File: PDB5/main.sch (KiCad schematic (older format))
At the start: 31 parts, among them P1 CONN_02X03, P4 CONN_01X02, P5 CONN_01X10, P6 CONN_01X10, P7 CONN_01X10, U1 PCA9698, U10 LTC6802-2, U11 LTC6802-2, U12 LTC6802-2, U13 LTC6802-2, U7 Littlebee, U8 Littlebee, U9 SC18IS602B

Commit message: test
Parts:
- removed P? (x3): CONN_01X03, symbol CONN_01X03
- removed R?: R, symbol R
- removed U10, U11, U12, U13: LTC6802-2, symbol LTC6802-2
- added C1: C, Capacitors_SMD:C_0805, symbol C
- added D1: ZENER, Diodes_SMD:SOD-123, symbol ZENER
- added D3: LED, LEDs:LED_0603, symbol LED
- added P10, P2, P3, P7, P8, P9: CONN_01X02, Pin_Headers:Pin_Header_Straight_1x02, symbol CONN_01X02
- added P15, P16: CONN_XT60_Female, KiCad-Dev:XT60, symbol CONN_XT60_Female
- added R2: R, Resistors_SMD:R_0603, symbol R
- added R3: R, symbol R
- C2: renamed from C?; footprint (none) -> SMD_Packages:SMD-2010_Pol
- C3: renamed from C?; footprint (none) -> Capacitors_SMD:C_0805
- D2: renamed from D?; footprint (none) -> LEDs:LED_0603
- D4: renamed from D?; footprint (none) -> Diodes_SMD:SOD-123
- P1: renamed from P?; footprint (none) -> Pin_Headers:Pin_Header_Straight_1x03
- P4, P5: renamed from P?; footprint (none) -> Pin_Headers:Pin_Header_Straight_1x02
- R1: renamed from R?; footprint (none) -> Resistors_SMD:R_0603
- U1: renamed from U9; footprint (none) -> Housings_SSOP:TSSOP-16_4.4x5mm_Pitch0.65mm
- gave numbers to parts that had none: 6
- renumbered P7 to P11, P4 to P12, P5 to P13, P6 to P14, P1 to P6, U1 to U2, U7 to U3, U8 to U4
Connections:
- net GPIO_Reset is gone; now on net RST: U2.56 (RESET)
- net +3V3: now also U1.12 (VDD), C1.1, D1.2 (A), R2.2, R3.1
- net ADC_1/SCL: now also P8.1 (P1)
- net ADC_1/SDA: now also P7.2 (P2)
- net ADC_2/SCL: now also P10.1 (P1)
- net ADC_2/SDA: now also P9.2 (P2)
- net GND: now also U1.14 (A0), U1.15 (A1), U1.16 (A2), U1.4 (VSS), U2.27 (AD0), U2.28 (AD1), U2.29 (AD2), C1.2, D1.1 (K), P15.1 (-), P16.1 (-)
- net SCL: now also P2.1 (P1), P7.1 (P1), P9.1 (P1)
- net SDA: now also P10.2 (P2), P3.2 (P2), P8.2 (P2)
- net pwr_mod_10/Power_Out: now also P16.2 (+)
- net pwr_mod_9/Power_Out: now also P15.2 (+)
- net RST: now reaches P6.4 (P4)
- net RST: now also U1.3 (RESET), R3.2
- net SS0: now reaches U1.1 (SS0)
- net SS2: now reaches U1.10 (SS2)
- net SCKI: now reaches U1.11 (SPICLK)
- net SS3: now reaches U1.13 (SS3)
- net SS1: now reaches U1.2 (SS1)
- net SDI: now reaches U1.5 (MOSI)
- net SDO: now reaches U1.6 (MISO)
- net at U1.7 (SDA): now also P3.1 (P1)
- net at U1.8 (SCL): now also P2.2 (P2)
- net at U1.9 (INT): now also D3.1 (K)
- new net: D3.2 (A), R2.1
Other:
- note removed: "Use header pin jumper to \nconfig the address"
- moved on the sheet: D2, P1, R1, U1

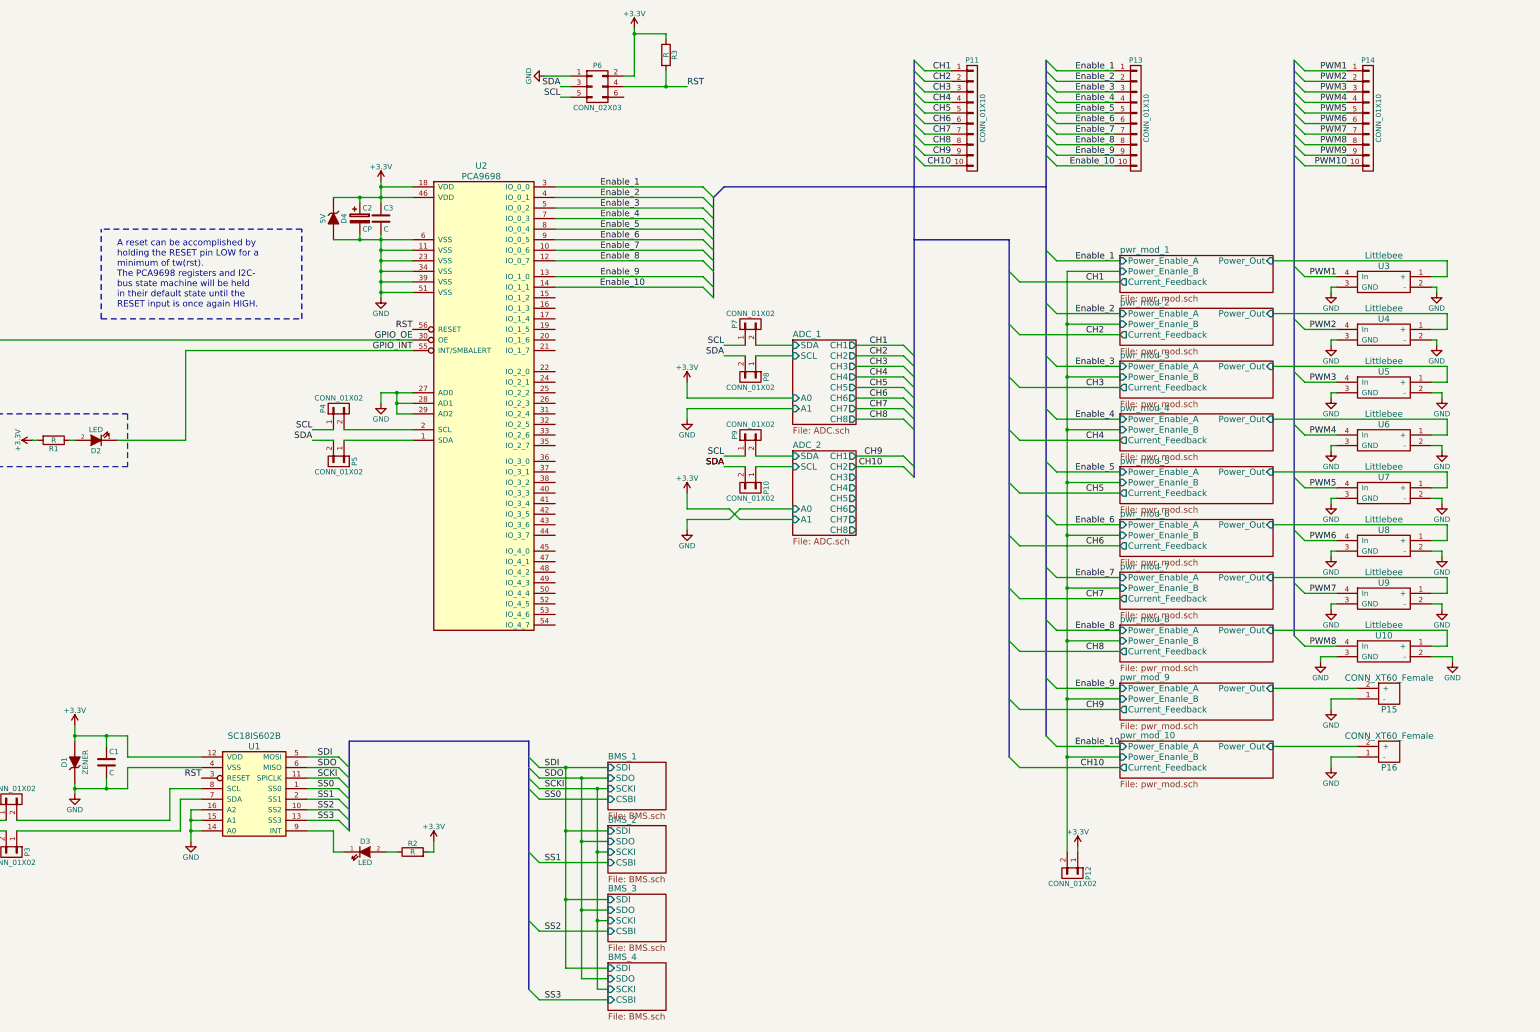
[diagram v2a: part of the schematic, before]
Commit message: test
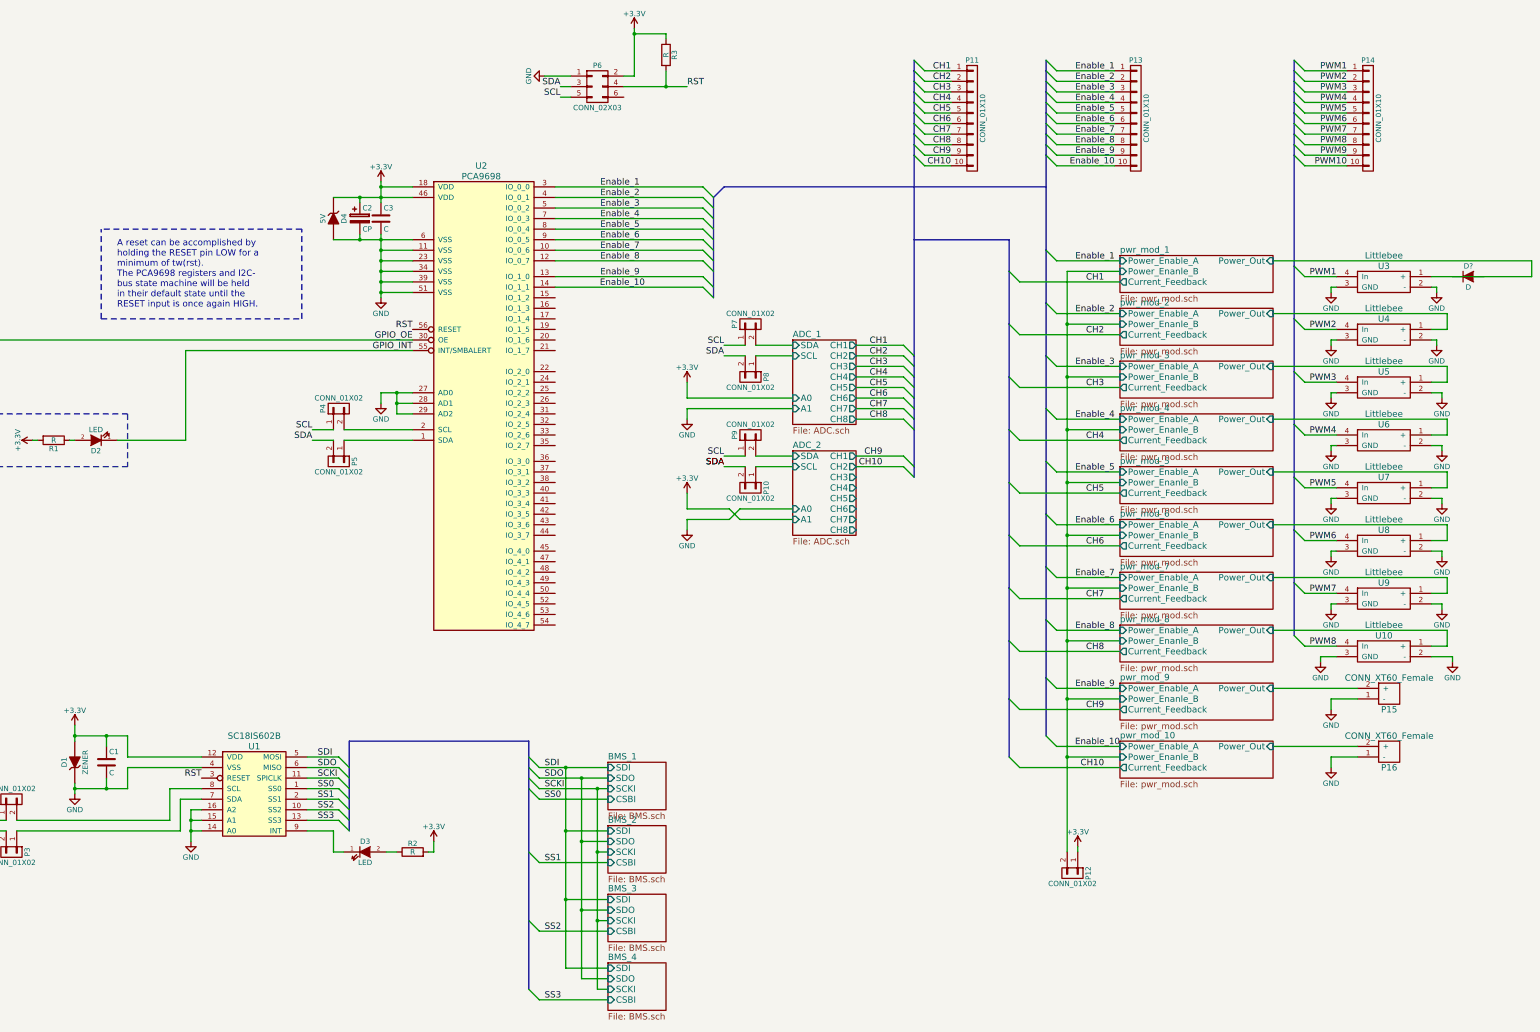
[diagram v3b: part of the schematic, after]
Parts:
- added D?: D, symbol D
